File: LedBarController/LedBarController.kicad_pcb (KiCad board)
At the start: 2 copper layers, 145.1 x 25 mm, 104 parts, among them J1005 ISP, J1101 Conn_01x02, J1201 Barrel_Jack_Switch, J1301 Screw_Terminal_01x03, J201 Female pitch strip 1x7 pins 2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, J202 Female 2x7 pins 2.0mm pitch, J203 Female pitch strip 1x7 pins 2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, J701 Male pitch strip 1x7 pins 2.0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, J702 Conn_01x05, J703 Conn_01x05, J801 Conn_01x05, J802 Male pitch strip 2x7pins 2.0m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, J803 Conn_01x05, J804 Conn_01x05, J805 Conn_01x05, J901 Male pitch strip 1x7 pins 2.0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, J902 Conn_01x05, J903 Conn_01x05, Q1201 FQP47P06, Q301 Si2302DS, Q302 Si2302DS, Q303 Si2302DS, Q304 Si2302DS, Q401 Si2302DS, Q402 Si2302DS, Q403 Si2302DS, Q404 Si2302DS, Q501 Si2302DS, Q502 Si2302DS, Q503 Si2302DS, Q504 Si2302DS, Q601 Si2302DS, Q602 Si2302DS, Q603 Si2302DS, Q604 Si2302DS, SW1001 reset, SW801 4x42.3mm PCB Tactile Push But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, U1001 ATmega328P-AU, U1101 LM358DR, U1201 AMS1117-5.0, U1202 INA219AxD, U1301 MAX485E, U201 PCA9685PW, Y1001 14.7456Mhz

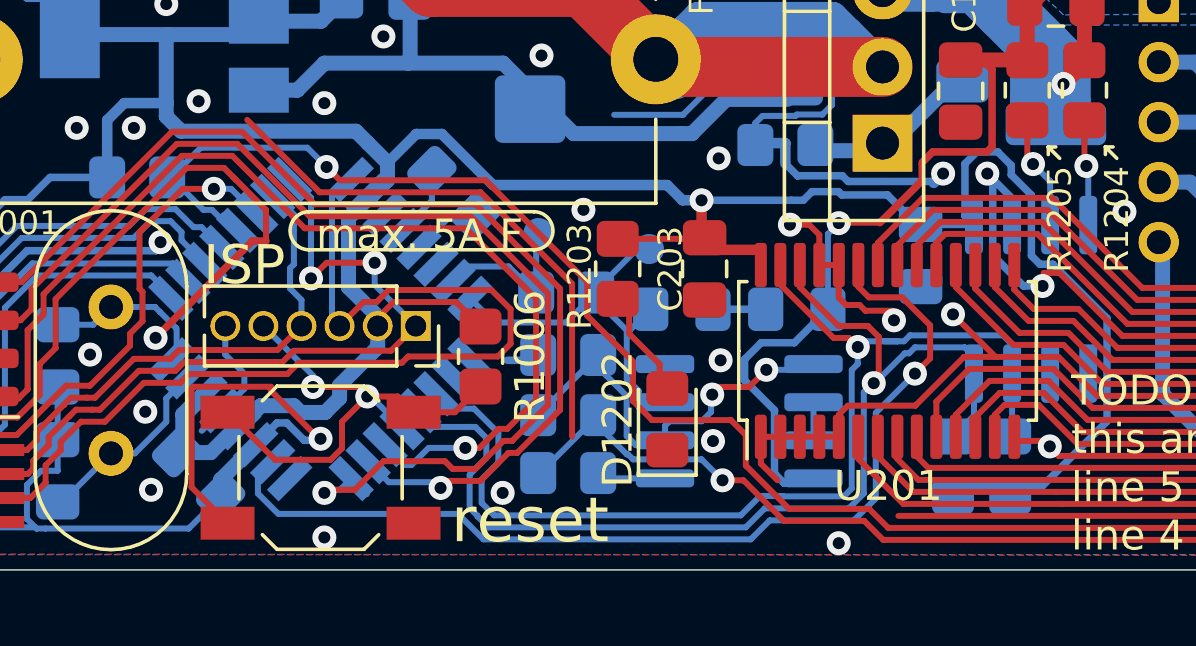
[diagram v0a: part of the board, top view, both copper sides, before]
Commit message: Improved ISP connector silk layer
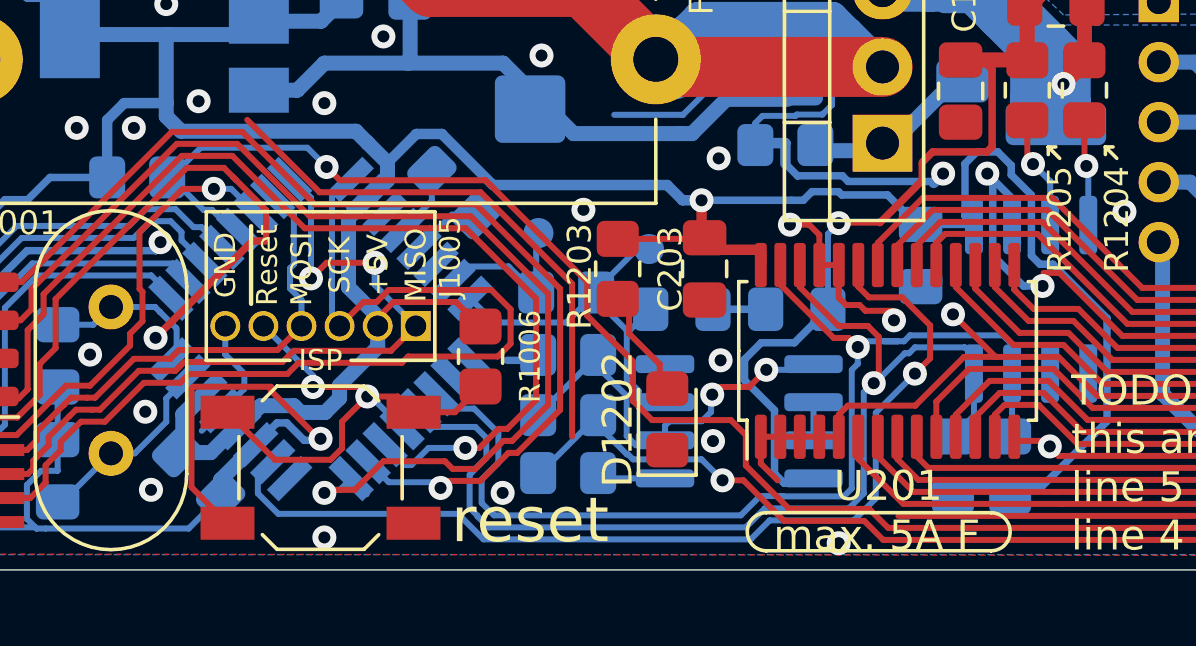
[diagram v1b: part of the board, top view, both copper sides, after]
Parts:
- J1005: footprint Connector_PinSocket_1.27mm:PinSocket_1x06_P1.27mm_Vertical -> LedBarController:ISP_P1.27mm_single_row
- moved J1005 6.35 mm to (52.3, 39.4), turned to 90 degrees
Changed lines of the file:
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@@
     (add_net /Power/surge_bypass)
   )
+  (module LedBarController:ISP_P1.27mm_single_row (layer F.Cu)
+    (at 52.324 39.37 90)
+    (descr "Through hole straight socket strip, 1x06, 1.27mm pitch, single row (from Kicad 4.0.7), script generated")
+    (tags "Through hole socket strip THT 1x06 1.27mm single row")
+    (fp_text reference J1005 (at 2.286 7.493 90) (layer F.SilkS)
+      (effects (font (size 0.7 0.7) (thickness 0.15)))
+    )
+    (fp_text value ISP (at 0 8.485 90) (layer F.Fab)
+      (effects (font (size 1 1) (thickness 0.15)))
+    )
+    (fp_text user ISP (at -1.143 3.175 180) (layer F.SilkS)
+      (effects (font (size 0.7 0.7) (thickness 0.15)))
+    )
+    (fp_text user SCK (at 2.032 3.81 90) (layer F.SilkS)
+      (effects (font (size 0.7 0.7) (thickness 0.15)))
+    )
+    (fp_text user %R (at 0 3.175) (layer F.Fab)
+      (effects (font (size 1 1) (thickness 0.15)))
+    )
+    (fp_line (start 3.81 -0.635) (end 3.81 6.985) (layer F.CrtYd) (width 0.05))
+    (fp_line (start -1.75 -1.15) (end 1.778 -1.15) (layer F.CrtYd) (width 0.05))
+    (fp_line (start -1.75 7.5) (end -1.75 -1.15) (layer F.CrtYd) (width 0.05))
+    (fp_line (start 1.778 7.5) (end -1.75 7.5) (layer F.CrtYd) (width 0.05))
+    (fp_line (start 1.27 -0.635) (end 1.27 6.985) (layer F.Fab) (width 0.1))
+    (fp_line (start -1.27 -0.635) (end 1.27 -0.635) (layer F.Fab) (width 0.1))
+    (fp_line (start -1.27 6.35) (end -1.27 -0.635) (layer F.Fab) (width 0.1))
+    (fp_line (start -0.635 6.985) (end -1.27 6.35) (layer F.Fab) (width 0.1))
+    (fp_line (start 1.27 6.985) (end -0.635 6.985) (layer F.Fab) (width 0.1))
+    (fp_line (start -1.143 2.159) (end -1.143 -0.635) (layer F.SilkS) (width 0.12))
+    (fp_line (start -1.143 -0.635) (end 3.81 -0.635) (layer F.SilkS) (width 0.12))
+    (fp_line (start 3.81 -0.635) (end 3.81 6.985) (layer F.SilkS) (width 0.12))
+    (fp_line (start 3.81 6.985) (end -1.143 6.985) (layer F.SilkS) (width 0.12))
+    (fp_line (start -1.143 6.985) (end -1.143 4.191) (layer F.SilkS) (width 0.12))
+    (fp_line (start 1.778 -1.143) (end 1.778 -0.635) (layer F.CrtYd) (width 0.05))
+    (fp_line (start 1.778 -0.635) (end 3.81 -0.635) (layer F.CrtYd) (width 0.05))
+    (fp_line (start 1.778 7.493) (end 1.778 6.985) (layer F.CrtYd) (width 0.05))
+    (fp_line (start 1.778 6.985) (end 3.81 6.985) (layer F.CrtYd) (width 0.05))
+    (fp_text user GND (at 2.032 0 90) (layer F.SilkS)
+      (effects (font (size 0.7 0.7) (thickness 0.15)))
+    )
+    (fp_text user ~Reset (at 2.032 1.397 90) (layer F.SilkS)
+      (effects (font (size 0.7 0.7) (thickness 0.15)))
+    )
+    (fp_text user MOSI (at 1.905 2.54 90) (layer F.SilkS)
+      (effects (font (size 0.7 0.7) (thickness 0.15)))
+    )
+    (fp_text user +5V (at 2.032 5.08 90) (layer F.SilkS)
+      (effects (font (size 0.7 0.7) (thickness 0.15)))
+    )
+    (fp_text user MISO (at 2.032 6.35 90) (layer F.SilkS)
+      (effects (font (size 0.7 0.7) (thickness 0.15)))
+    )
+    (pad 6 thru_hole oval (at 0 0 270) (size 1 1) (drill 0.7) (layers *.Cu *.Mask)
+      (net 1 GND))
+    (pad 5 thru_hole oval (at 0 1.27 270) (size 1 1) (drill 0.7) (layers *.Cu *.Mask)
+      (net 74 /Microcontroller/reset))
+    (pad 4 thru_hole oval (at 0 2.54 270) (size 1 1) (drill 0.7) (layers *.Cu *.Mask)
+      (net 75 /Microcontroller/isp_mosi))
+    (pad 3 thru_hole oval (at 0 3.81 270) (size 1 1) (drill 0.7) (layers *.Cu *.Mask)
+      (net 76 /Microcontroller/isp_sck))
+    (pad 2 thru_hole oval (at 0 5.08 270) (size 1 1) (drill 0.7) (layers *.Cu *.Mask)
+      (net 3 +5V))
+    (pad 1 thru_hole rect (at 0 6.35 270) (size 1 1) (drill 0.7) (layers *.Cu *.Mask)
+      (net 77 /Microcontroller/isp_miso))
+    (model ${KISYS3DMOD}/Connector_PinSocket_1.27mm.3dshapes/PinSocket_1x06_P1.27mm_Vertical.wrl
+      (at (xyz 0 0 0))
+      (scale (xyz 1 1 1))
+      (rotate (xyz 0 0 0))
+    )
+  )
   (module Diode_SMD:D_SMB_Handsoldering (layer B.Cu)
     (at 30.607 30.734 270)
@@
       (effects (font (size 0.8 0.8) (thickness 0.15)))
     )
-    (fp_text value "max. 5A F" (at 7.874 -5.842) (layer F.SilkS)
+    (fp_text value "max. 5A F" (at -7.366 -15.875) (layer F.SilkS)
       (effects (font (size 1 1) (thickness 0.15)))
     )
@@
     )
   )
-  (module Connector_PinSocket_1.27mm:PinSocket_1x06_P1.27mm_Vertical (layer F.Cu)
-    (at 58.674 39.37 270)
-    (descr "Through hole straight socket strip, 1x06, 1.27mm pitch, single row (from Kicad 4.0.7), script generated")
-    (tags "Through hole socket strip THT 1x06 1.27mm single row")
-    (fp_text reference J1005 (at -1.778 3.429 180) (layer F.Fab)
-      (effects (font (size 1 1) (thickness 0.15)))
-    )
-    (fp_text value ISP (at -2.032 5.715 180) (layer F.SilkS)
-      (effects (font (size 1.3 1.3) (thickness 0.15)))
-    )
-    (fp_line (start -1.8 7.5) (end -1.8 -1.15) (layer F.CrtYd) (width 0.05))
-    (fp_line (start 1.75 7.5) (end -1.8 7.5) (layer F.CrtYd) (width 0.05))
-    (fp_line (start 1.75 -1.15) (end 1.75 7.5) (layer F.CrtYd) (width 0.05))
-    (fp_line (start -1.8 -1.15) (end 1.75 -1.15) (layer F.CrtYd) (width 0.05))
-    (fp_line (start 0 -0.76) (end 1.33 -0.76) (layer F.SilkS) (width 0.12))
-    (fp_line (start 1.33 -0.76) (end 1.33 0) (layer F.SilkS) (width 0.12))
-    (fp_line (start 1.33 0.635) (end 1.33 7.045) (layer F.SilkS) (width 0.12))
-    (fp_line (start 0.30753 7.045) (end 1.33 7.045) (layer F.SilkS) (width 0.12))
-    (fp_line (start -1.33 7.045) (end -0.30753 7.045) (layer F.SilkS) (width 0.12))
-    (fp_line (start -1.33 0.635) (end -1.33 7.045) (layer F.SilkS) (width 0.12))
-    (fp_line (start 0.76 0.635) (end 1.33 0.635) (layer F.SilkS) (width 0.12))
-    (fp_line (start -1.33 0.635) (end -0.76 0.635) (layer F.SilkS) (width 0.12))
-    (fp_line (start -1.27 6.985) (end -1.27 -0.635) (layer F.Fab) (width 0.1))
-    (fp_line (start 1.27 6.985) (end -1.27 6.985) (layer F.Fab) (width 0.1))
-    (fp_line (start 1.27 0) (end 1.27 6.985) (layer F.Fab) (width 0.1))
-    (fp_line (start 0.635 -0.635) (end 1.27 0) (layer F.Fab) (width 0.1))
-    (fp_line (start -1.27 -0.635) (end 0.635 -0.635) (layer F.Fab) (width 0.1))
-    (fp_text user %R (at 0 3.175) (layer F.Fab)
-      (effects (font (size 1 1) (thickness 0.15)))
-    )
-    (pad 6 thru_hole oval (at 0 6.35 270) (size 1 1) (drill 0.7) (layers *.Cu *.Mask)
-      (net 1 GND))
-    (pad 5 thru_hole oval (at 0 5.08 270) (size 1 1) (drill 0.7) (layers *.Cu *.Mask)
-      (net 74 /Microcontroller/reset))
-    (pad 4 thru_hole oval (at 0 3.81 270) (size 1 1) (drill 0.7) (layers *.Cu *.Mask)
-      (net 75 /Microcontroller/isp_mosi))
-    (pad 3 thru_hole oval (at 0 2.54 270) (size 1 1) (drill 0.7) (layers *.Cu *.Mask)
-      (net 76 /Microcontroller/isp_sck))
-    (pad 2 thru_hole oval (at 0 1.27 270) (size 1 1) (drill 0.7) (layers *.Cu *.Mask)
-      (net 3 +5V))
-    (pad 1 thru_hole rect (at 0 0 270) (size 1 1) (drill 0.7) (layers *.Cu *.Mask)
-      (net 77 /Microcontroller/isp_miso))
-    (model ${KISYS3DMOD}/Connector_PinSocket_1.27mm.3dshapes/PinSocket_1x06_P1.27mm_Vertical.wrl
-      (at (xyz 0 0 0))
-      (scale (xyz 1 1 1))
-      (rotate (xyz 0 0 0))
-    )
-  )
   (module Capacitor_THT:CP_Radial_D13.0mm_P5.00mm (layer F.Cu)
     (at 91.44 29.718 270)
@@
     (attr smd)
     (fp_text reference R1006 (at 0 -1.65 90) (layer F.SilkS)
-      (effects (font (size 1 1) (thickness 0.15)))
+      (effects (font (size 0.7 0.7) (thickness 0.15)))
     )
     (fp_text value 10k (at 0 1.65 90) (layer F.Fab)
@@
     )
   )
-  (gr_line (start 62.611 35.56) (end 55.118 35.56) (layer F.SilkS) (width 0.12))
-  (gr_line (start 55.118 36.83) (end 62.611 36.83) (layer F.SilkS) (width 0.12))
-  (gr_arc (start 55.118 36.195) (end 55.118 35.56) (angle -180) (layer F.SilkS) (width 0.12))
-  (gr_arc (start 62.611 36.195) (end 62.611 36.83) (angle -180) (layer F.SilkS) (width 0.12))
+  (gr_line (start 77.851 45.593) (end 70.358 45.593) (layer F.SilkS) (width 0.12))
+  (gr_line (start 70.358 46.863) (end 77.851 46.863) (layer F.SilkS) (width 0.12))
+  (gr_arc (start 70.358 46.228) (end 70.358 45.593) (angle -180) (layer F.SilkS) (width 0.12))
+  (gr_arc (start 77.851 46.228) (end 77.851 46.863) (angle -180) (layer F.SilkS) (width 0.12))
   (gr_line (start 42.545 42.926) (end 42.291 42.926) (layer F.SilkS) (width 0.12))
   (gr_line (start 42.545 42.926) (end 42.799 43.18) (layer F.SilkS) (width 0.12))
@@
   (segment (start 55.7007 37.2618) (end 55.18 37.7825) (width 0.2) (layer F.Cu) (net 77))
   (segment (start 57.3024 37.2618) (end 55.7007 37.2618) (width 0.2) (layer F.Cu) (net 77))
-  (segment (start 57.3024 37.9984) (end 58.674 39.37) (width 0.2) (layer B.Cu) (net 77))
-  (segment (start 57.3024 37.2618) (end 57.3024 37.9984) (width 0.2) (layer B.Cu) (net 77))
   (segment (start 45.739 44.304) (end 45.173 44.304) (width 0.2) (layer F.Cu) (net 77))
   (segment (start 45.923001 44.119999) (end 45.739 44.304) (width 0.2) (layer F.Cu) (net 77))
@@
   (segment (start 49.441688 40.863711) (end 50.658289 40.863711) (width 0.2) (layer F.Cu) (net 77))
   (segment (start 50.7775 40.7445) (end 50.65829 40.863711) (width 0.2) (layer F.Cu) (net 77))
+  (segment (start 57.3024 37.9984) (end 58.674 39.37) (width 0.2) (layer B.Cu) (net 77))
+  (segment (start 57.3024 37.2618) (end 57.3024 37.9984) (width 0.2) (layer B.Cu) (net 77))
   (segment (start 42.10799 42.64119) (end 42.1016 42.6348) (width 0.2) (layer B.Cu) (net 78))
   (segment (start 42.605789 42.64119) (end 42.10799 42.64119) (width 0.2) (layer B.Cu) (net 78))

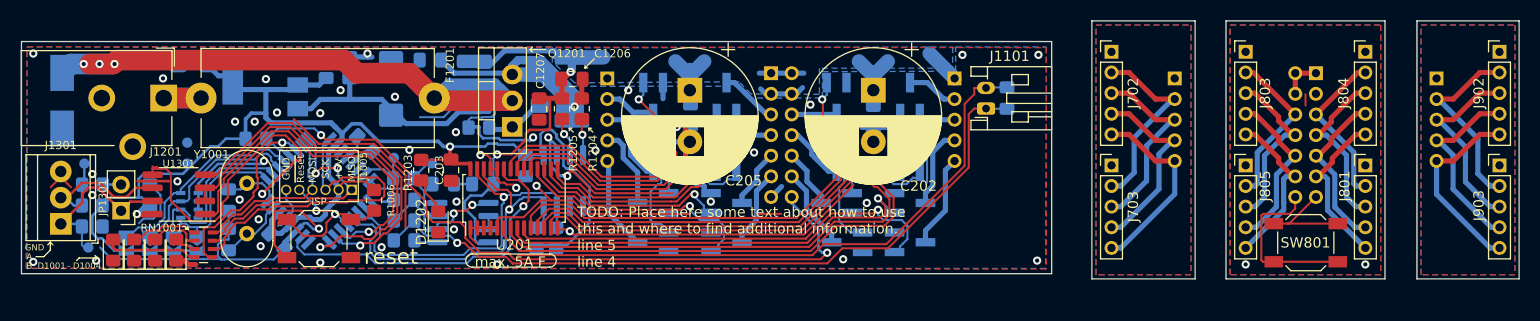
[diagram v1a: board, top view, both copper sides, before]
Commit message: Added AT24C256
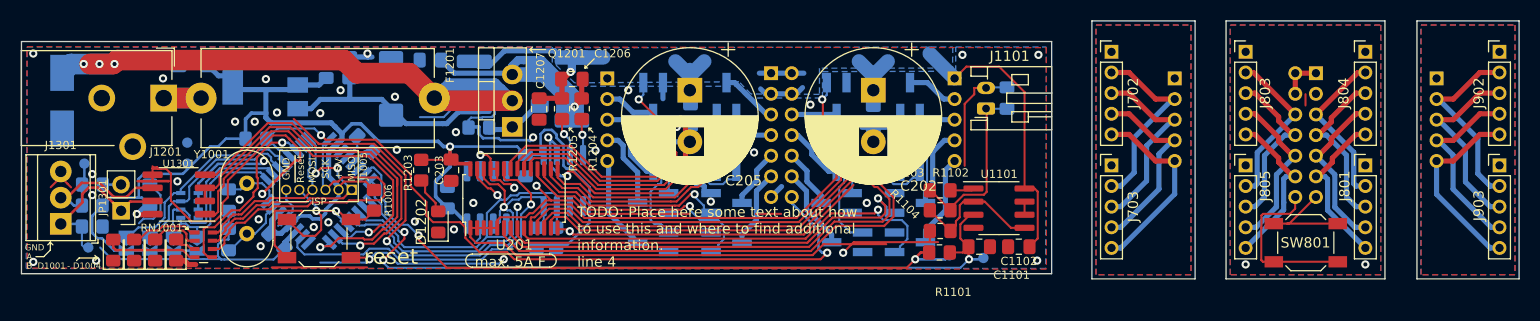
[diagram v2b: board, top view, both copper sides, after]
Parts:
- added C1005: 0.1uF, Capacitor_SMD:C_0805_2012Metric_Pad1.18x1.45mm_HandSolder, B.Cu at (67.9, 40.1)
- added U1002: AT24C256, Package_SO:SOP-8_3.76x4.96mm_P1.27mm, B.Cu at (71.8, 40.1)
- C1101, C1102, R1101, R1102, R1103, R1104, U1101: moved to F.Cu
- moved TP1102 54.6 mm to (116.6, 45.7)
- moved TP1101 54.2 mm to (119.9, 46.0)
- moved R1101 52.4 mm to (115.6, 45.4)
- moved C1101 52.3 mm to (119.5, 44.9)
- moved C1102 52.3 mm to (123.3, 44.9)
- moved R1102 52.2 mm to (115.7, 39.4)
- moved R1104 52.0 mm to (115.7, 43.4)
- moved U1101 52.0 mm to (121.4, 41.1)
- moved R1103 52.0 mm to (115.7, 41.4)
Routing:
- net /Microcontroller/0_10v_ain_1: track 14.7 -> 76.6 mm, vias 0 -> 3
- net /Microcontroller/0_10v_dout_1: track 5.13 -> 65.2 mm, vias 0 -> 2
- net Net-(C1104-Pad2): track 71.7 -> 17.3 mm, vias 1 -> 0
- net GND: track 326.3 -> 374.8 mm, vias 45 -> 48
- net +5V: track 138.6 -> 148.0 mm
- net Net-(R1103-Pad1): track 15.4 -> 13.2 mm, vias 2 -> 0
- net /Microcontroller/sda: track 36.1 -> 34.8 mm
- net VDD: track 70.4 -> 71.5 mm, vias 2 -> 1
- net Net-(R1102-Pad2): track 2.87 -> 2.30 mm
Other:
- board text added: "TODO: Move 0-10V circuit to the most right on the board. So we might add the AT24C256 anyway"
- board text added: "TODO: No copper on the Back where it could touch the aluminum profile! TODO: Make customized footprint to connect GRB(W) strips. (e.g. compatible with GRB)"
- board text added: "TODO: Place here some text about how to use this and where to find additional information. line 4"
- board text removed: "TODO: No copper on the Back where it could touch the aluminum profile! TODO: Make customized footprint to connect GRB(W) strips. (e.g. compatible with GRB) TODO: Make single row ISP connector, with silklayer explaining the pinout"
- board text removed: "TODO: Place here some text about how to use this and where to find additional information. line 5 line 4"
